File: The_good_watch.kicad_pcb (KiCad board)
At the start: 2 copper layers, 45 x 45 mm, 53 parts, among them IC1 DW01A, J1 Main, J2 USB_C_Receptacle_USB2.0, J3 PROG, J4 Screen, J5 Button, J6 Conn_02x07_Counter_Clockwise, M1 Motor_DC, Q1 FS8205A, Q2 LP0404N3T5G, SW1 SW_Push, SW2 SW_Push, SW3 SW_SPDT, U1 Opamp_Dual, U2 ESP32-WROOM, U3 TP4056, U4 TPS61200DRC

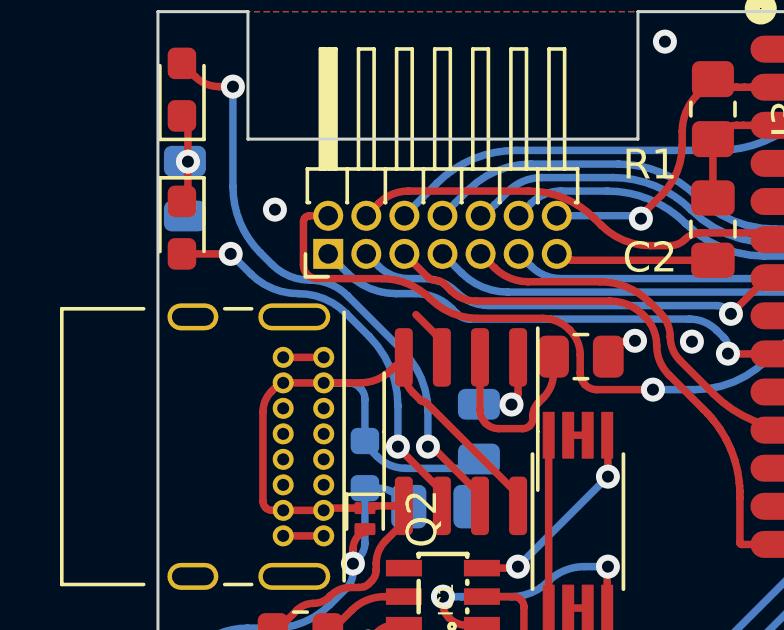
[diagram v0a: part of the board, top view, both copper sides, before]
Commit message: Fixed connector problems
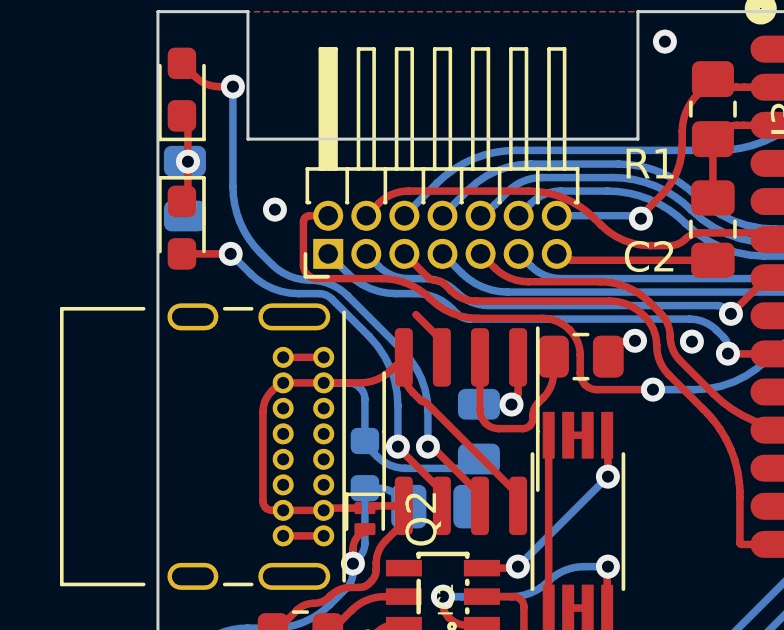
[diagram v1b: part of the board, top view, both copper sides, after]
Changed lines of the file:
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@@
   (arc (start 108 64.512307) (mid 108.002261 64.523677) (end 108.008702 64.533316) (width 0.25) (layer "F.Cu") (net 15))
   (arc (start 109.29339 65.818004) (mid 109.4204 66.008087) (end 109.465 66.232307) (width 0.25) (layer "F.Cu") (net 15))
-  (segment (start 107.039983 60.824647) (end 106.275311 60.059975) (width 0.25) (layer "B.Cu") (net 15))
+  (segment (start 107.039983 60.824647) (end 105.792884 59.577548) (width 0.25) (layer "B.Cu") (net 15))
   (segment (start 108 63.142332) (end 108 64.5) (width 0.25) (layer "B.Cu") (net 15))
+  (segment (start 104.683148 59.40048) (end 105.365453 59.400495) (width 0.25) (layer "B.Cu") (net 15))
   (segment (start 102.425 58.075) (end 103.090984 58.740984) (width 0.25) (layer "B.Cu") (net 15))
-  (arc (start 104.683148 59.40048) (mid 105.54482 59.571877) (end 106.275311 60.059975) (width 0.25) (layer "B.Cu") (net 15))
+  (arc (start 105.365453 59.400495) (mid 105.596777 59.446512) (end 105.792884 59.577548) (width 0.25) (layer "B.Cu") (net 15))
   (arc (start 103.090984 58.740984) (mid 103.821475 59.229082) (end 104.683148 59.40048) (width 0.25) (layer "B.Cu") (net 15))
   (arc (start 108 63.142332) (mid 107.750499 61.88801) (end 107.039983 60.824647) (width 0.25) (layer "B.Cu") (net 15))
